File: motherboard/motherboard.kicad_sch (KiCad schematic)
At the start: 60 parts, among them U1 MPR121QR2, U2 cap_touch, U23 cap_touch, U24 cap_touch, U25 cap_touch, U26 cap_touch, U27 cap_touch, U28 cap_touch, U29 cap_touch, U3 cap_touch, U30 cap_touch, U31 cap_touch, U32 cap_touch, U33 cap_touch, U34 cap_touch, U35 cap_touch, U36 cap_touch, U37 cap_touch

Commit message: mothrboard_ft
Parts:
- C1, C12, C13, C2, C5, C9: footprint Capacitor_Tantalum_SMD:CP_EIA-3528-12_Kemet-T_Pad1.50x2.35mm_HandSolder -> Capacitor_Tantalum_SMD:CP_EIA-1608-08_AVX-J_Pad1.25x1.05mm_HandSolder
- klr1, ktb1, ljlr1, ljtb1, rjlr2, rjtb1: footprint Package_TO_SOT_SMD:SOT-23 -> Package_TO_SOT_THT:TO-92S
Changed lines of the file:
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@@
 			)
 		)
-		(property "Footprint" "Package_TO_SOT_SMD:SOT-23"
+		(property "Footprint" "Package_TO_SOT_THT:TO-92S"
 			(at 143.51 44.45 0)
 			(effects
@@
 			)
 		)
-		(property "Footprint" "Capacitor_Tantalum_SMD:CP_EIA-3528-12_Kemet-T_Pad1.50x2.35mm_HandSolder"
+		(property "Footprint" "Capacitor_Tantalum_SMD:CP_EIA-1608-08_AVX-J_Pad1.25x1.05mm_HandSolder"
 			(at 63.1952 49.53 0)
 			(effects
@@
 			)
 		)
-		(property "Footprint" "Capacitor_Tantalum_SMD:CP_EIA-3528-12_Kemet-T_Pad1.50x2.35mm_HandSolder"
+		(property "Footprint" "Capacitor_Tantalum_SMD:CP_EIA-1608-08_AVX-J_Pad1.25x1.05mm_HandSolder"
 			(at 135.5852 49.53 0)
 			(effects
@@
 			)
 		)
-		(property "Footprint" "Capacitor_Tantalum_SMD:CP_EIA-3528-12_Kemet-T_Pad1.50x2.35mm_HandSolder"
+		(property "Footprint" "Capacitor_Tantalum_SMD:CP_EIA-1608-08_AVX-J_Pad1.25x1.05mm_HandSolder"
 			(at 98.7552 50.8 0)
 			(effects
@@
 			)
 		)
-		(property "Footprint" "Package_TO_SOT_SMD:SOT-23"
+		(property "Footprint" "Package_TO_SOT_THT:TO-92S"
 			(at 252.73 44.45 0)
 			(effects
@@
 			)
 		)
-		(property "Footprint" "Package_TO_SOT_SMD:SOT-23"
+		(property "Footprint" "Package_TO_SOT_THT:TO-92S"
 			(at 106.68 44.45 0)
 			(effects
@@
 			)
 		)
-		(property "Footprint" "Capacitor_Tantalum_SMD:CP_EIA-3528-12_Kemet-T_Pad1.50x2.35mm_HandSolder"
+		(property "Footprint" "Capacitor_Tantalum_SMD:CP_EIA-1608-08_AVX-J_Pad1.25x1.05mm_HandSolder"
 			(at 207.9752 49.53 0)
 			(effects
@@
 			)
 		)
-		(property "Footprint" "Package_TO_SOT_SMD:SOT-23"
+		(property "Footprint" "Package_TO_SOT_THT:TO-92S"
 			(at 215.9 44.45 0)
 			(effects
@@
 			)
 		)
-		(property "Footprint" "Package_TO_SOT_SMD:SOT-23"
+		(property "Footprint" "Package_TO_SOT_THT:TO-92S"
 			(at 180.34 44.45 0)
 			(effects
@@
 			)
 		)
-		(property "Footprint" "Package_TO_SOT_SMD:SOT-23"
+		(property "Footprint" "Package_TO_SOT_THT:TO-92S"
 			(at 71.12 44.45 0)
 			(effects
@@
 			)
 		)
-		(property "Footprint" "Capacitor_Tantalum_SMD:CP_EIA-3528-12_Kemet-T_Pad1.50x2.35mm_HandSolder"
+		(property "Footprint" "Capacitor_Tantalum_SMD:CP_EIA-1608-08_AVX-J_Pad1.25x1.05mm_HandSolder"
 			(at 172.4152 49.53 0)
 			(effects
@@
 			)
 		)
-		(property "Footprint" "Capacitor_Tantalum_SMD:CP_EIA-3528-12_Kemet-T_Pad1.50x2.35mm_HandSolder"
+		(property "Footprint" "Capacitor_Tantalum_SMD:CP_EIA-1608-08_AVX-J_Pad1.25x1.05mm_HandSolder"
 			(at 244.8052 49.53 0)
 			(effects

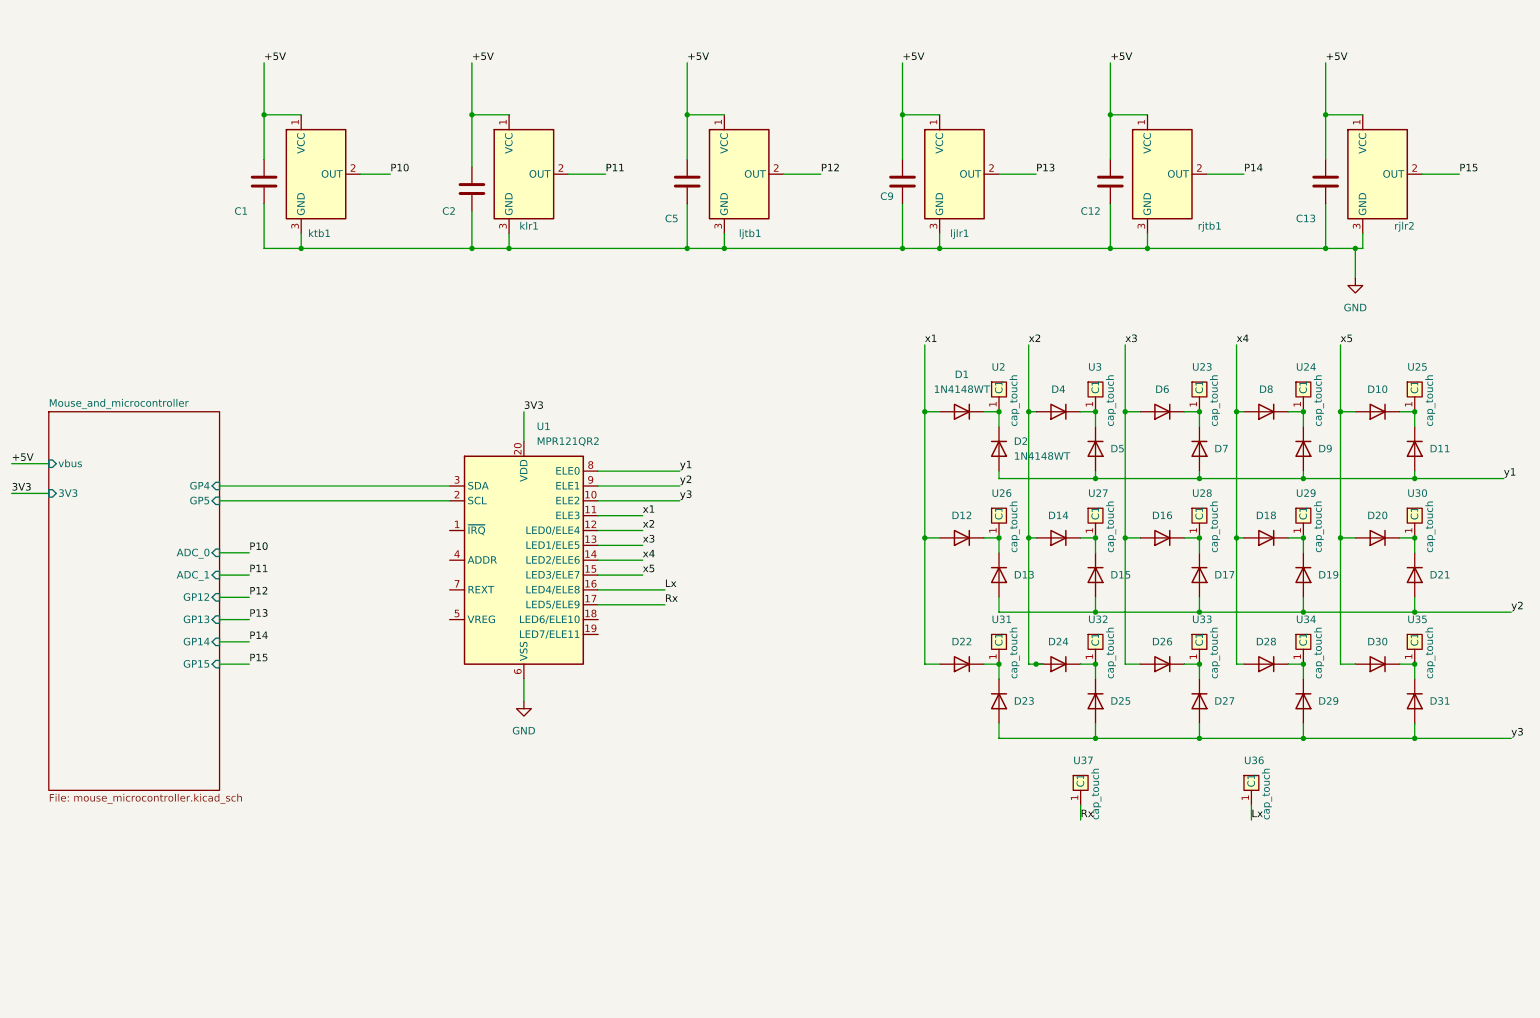
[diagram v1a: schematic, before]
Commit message: two_will
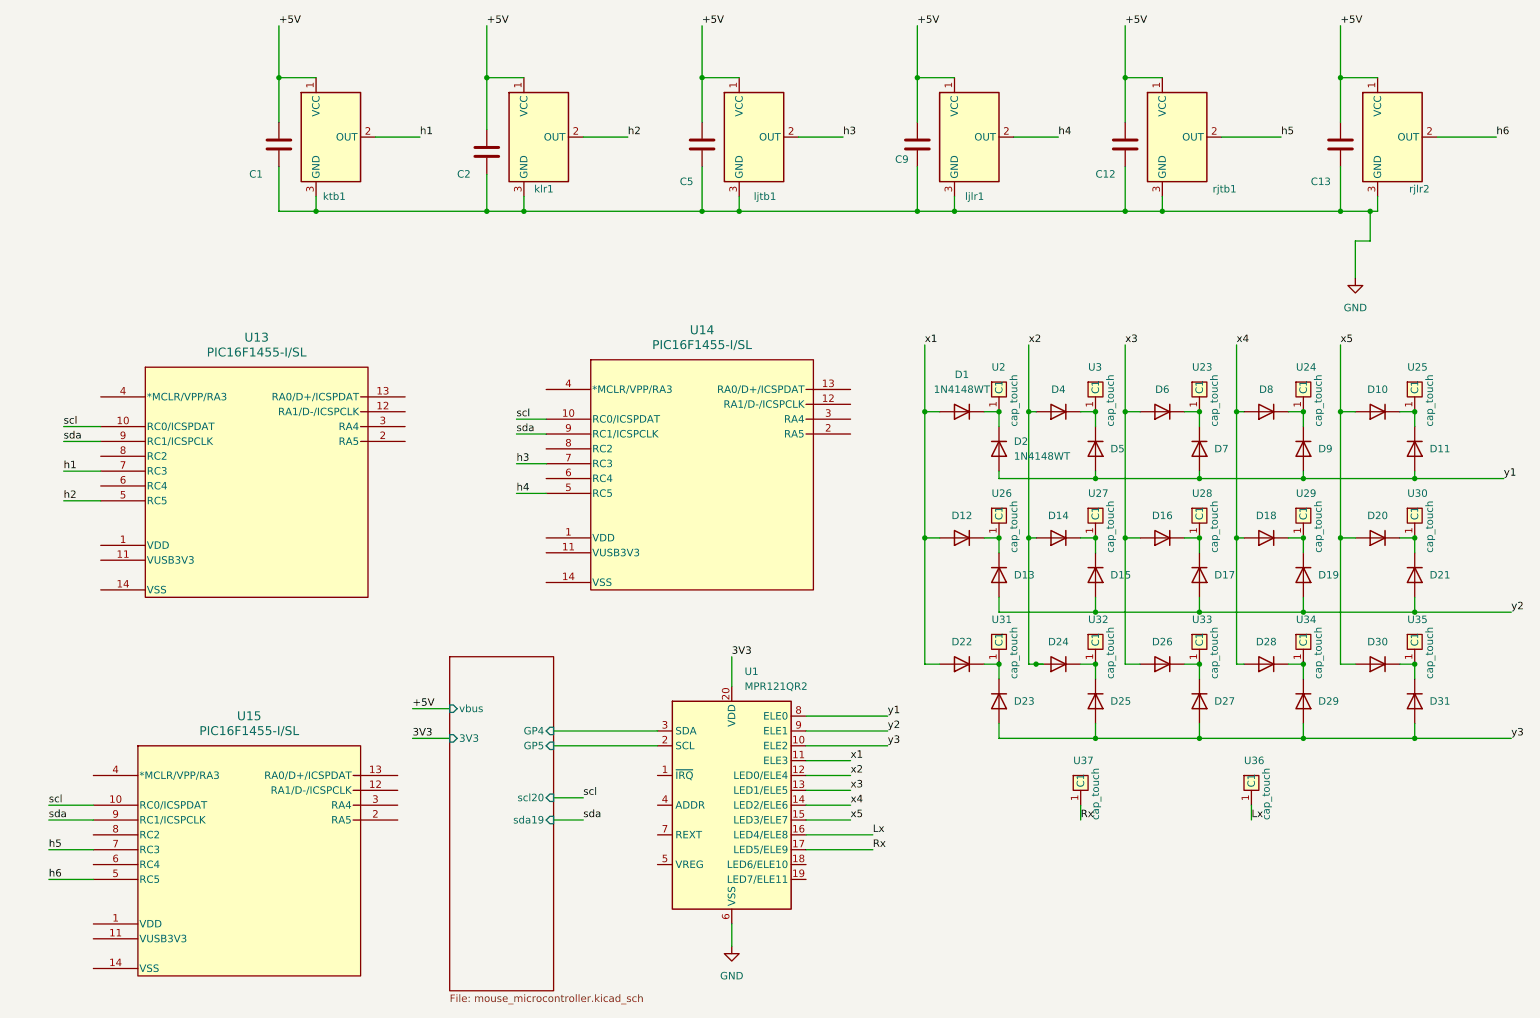
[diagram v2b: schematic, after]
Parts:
- added U13, U14, U15: PIC16F1455-I/SL, 42QT1481:SOIC14_SL_MCH, symbol touch_keys:PIC16F1455-I_SL
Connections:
- net P10 renamed h1
- net h1: now also U13.7 (RC3)
- net P11 renamed h2
- net h2: now also U13.5 (RC5)
- net P12 renamed h3
- net h3: now also U14.7 (RC3)
- net P13 renamed h4
- net h4: now also U14.5 (RC5)
- net P14 renamed h5
- net h5: now also U15.7 (RC3)
- net P15 renamed h6
- net h6: now also U15.5 (RC5)
- new net scl: U13.10 (RC0/ICSPDAT), U14.10 (RC0/ICSPDAT), U15.10 (RC0/ICSPDAT)
- new net sda: U13.9 (RC1/ICSPCLK), U14.9 (RC1/ICSPCLK), U15.9 (RC1/ICSPCLK)
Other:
- sheet Mouse_and_microcontroller ports: added scl20, sda19; removed ADC_0, ADC_1, GP12, GP13, GP14, GP15
- moved on the sheet: C1, C12, C13, C2, C5, C9, U1, klr1, ktb1, ljlr1, ljtb1, rjlr2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
